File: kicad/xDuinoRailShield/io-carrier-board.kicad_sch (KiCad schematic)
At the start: 8 parts, among them J1 Screw_Terminal_01x02, U7 MOUDLE-SEEEDUINO-XIAO-ESP32C3

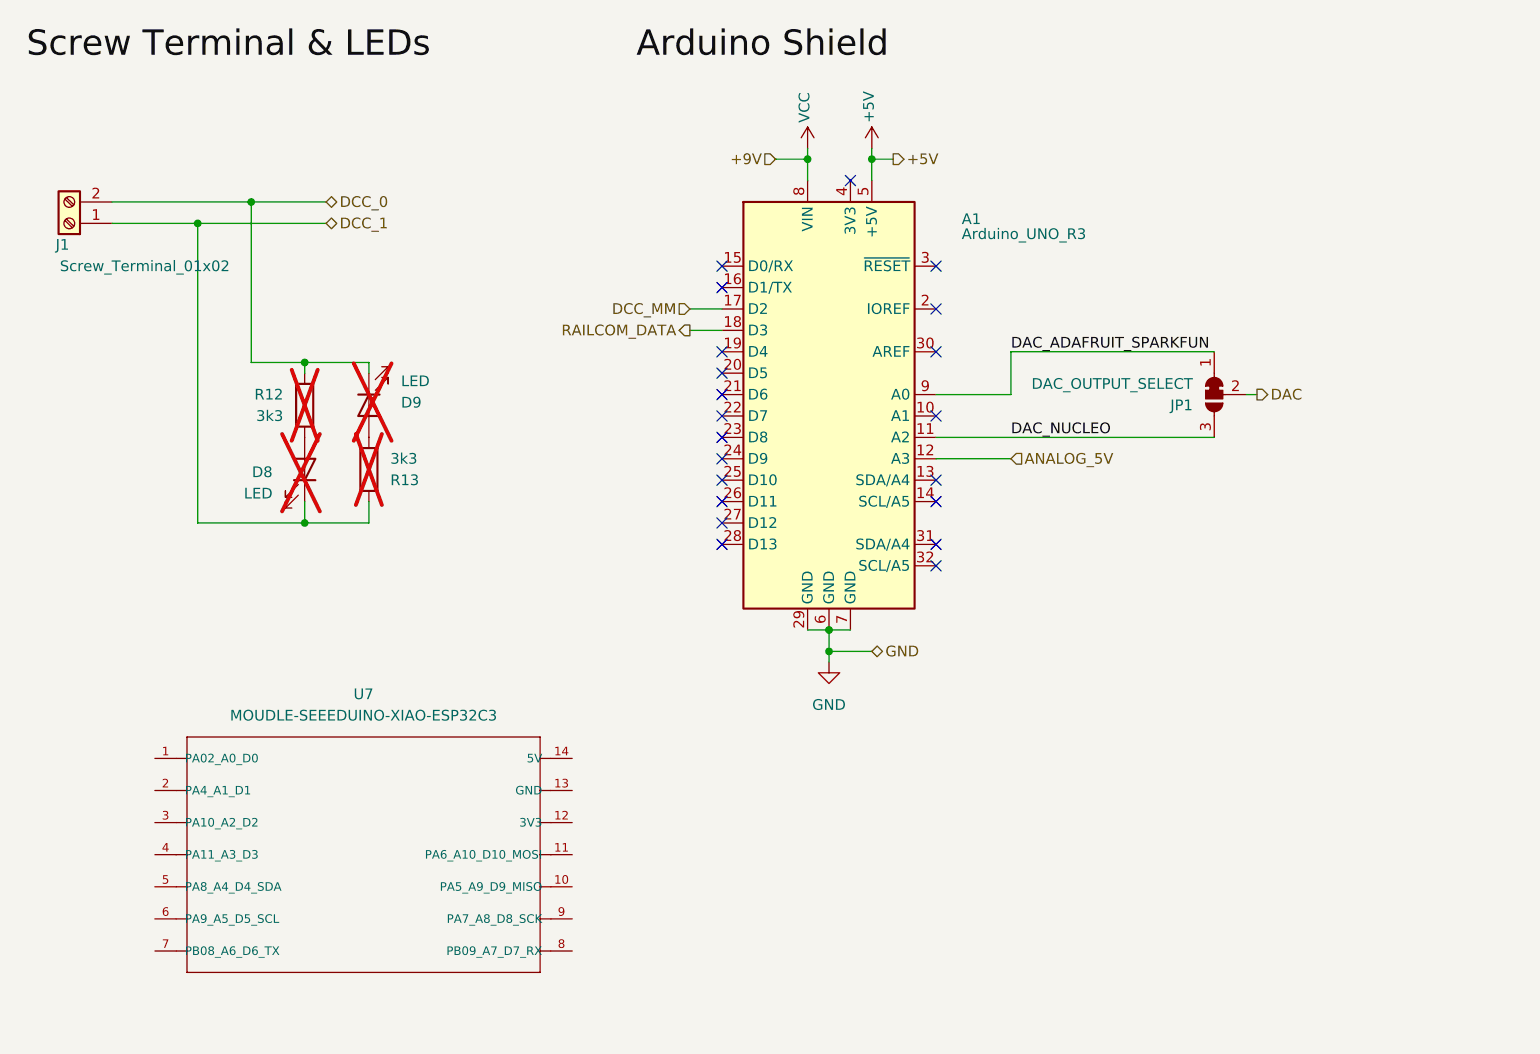
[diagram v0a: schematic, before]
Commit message: More nice changes
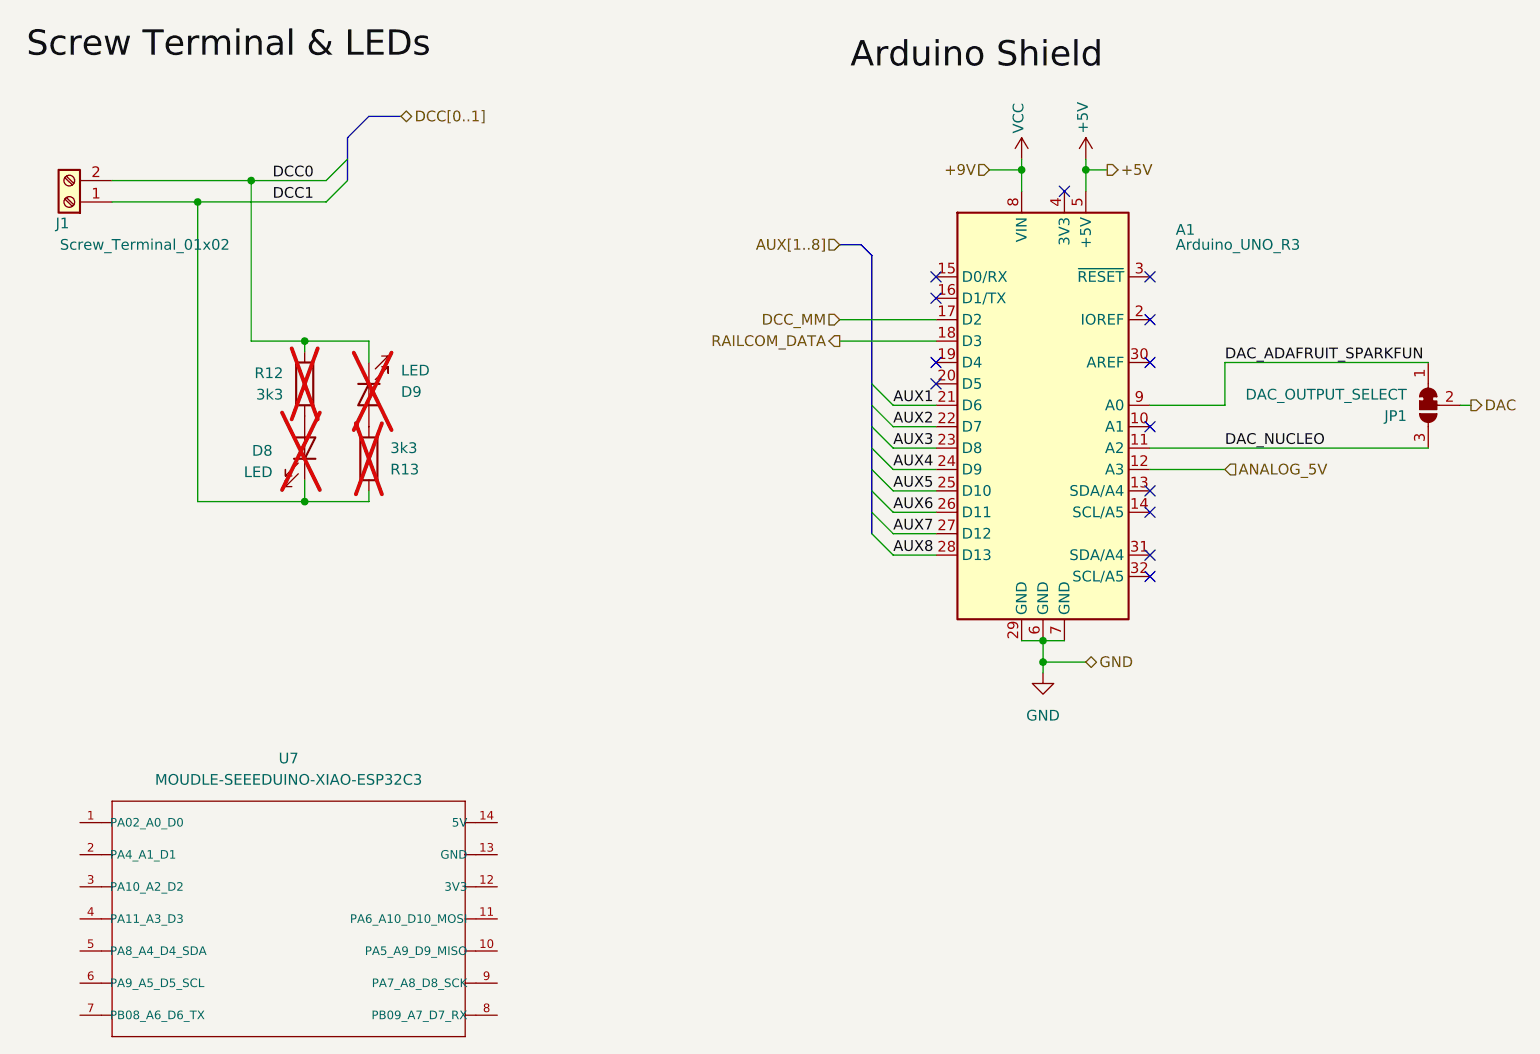
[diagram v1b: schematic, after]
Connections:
- net AUX1: now reaches A1.21 (D6)
- net AUX2: now reaches A1.22 (D7)
- net AUX3: now reaches A1.23 (D8)
- net AUX4: now reaches A1.24 (D9)
- net AUX5: now reaches A1.25 (D10)
- net AUX6: now reaches A1.26 (D11)
- net AUX7: now reaches A1.27 (D12)
- net AUX8: now reaches A1.28 (D13)
- net DCC_0 renamed DCC0
- net DCC_1 renamed DCC1
- no-connect marks 21 -> 13
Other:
- moved on the sheet: A1, D8, D9, J1, JP1, R12, R13, U7
